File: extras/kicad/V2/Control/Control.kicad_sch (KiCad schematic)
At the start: 41 parts, among them J1 Ultrasonic Ranging, J2 Conn_01x05, J3 Output, J4 Input, J6 left, J7 right, P8 BeagleBone_Black_Header, P9 BeagleBone_Black_Header, U1 SparkFun-micromod, U2 ESP-01-WIFI, U3 LIS3DHTR, U4 BNO085-breackout, U6 PCA9557PW

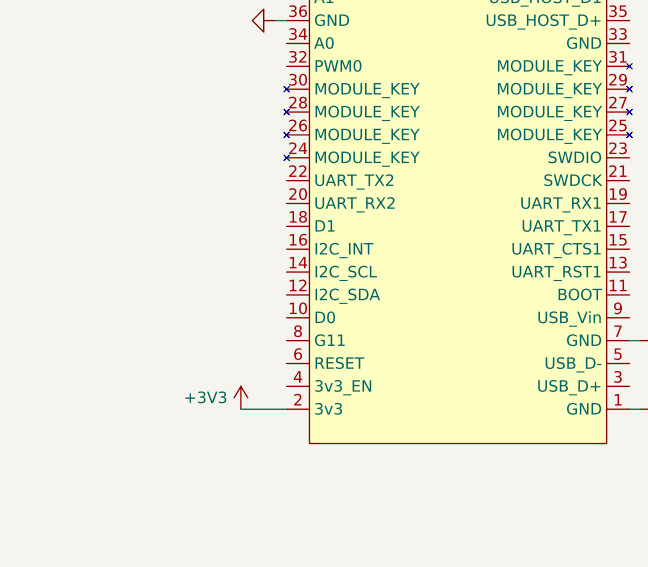
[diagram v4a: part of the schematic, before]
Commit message: f
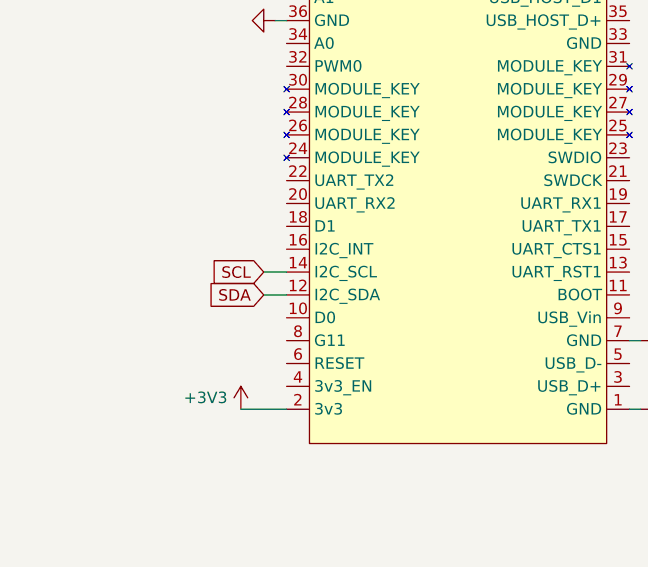
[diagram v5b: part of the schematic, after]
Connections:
- net SCL: now also U1.14 (I2C_SCL)
- net SDA: now also U1.12 (I2C_SDA)
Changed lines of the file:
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@@
+    (stroke (width 0) (type default) (color 0 0 0 0))
+  )
+  (wire (pts (xy 53.34 130.81) (xy 50.8 130.81))
     (stroke (width 0) (type default) (color 0 0 0 0))
   )
@@
   )
   (wire (pts (xy 189.23 102.87) (xy 193.04 102.87))
+    (stroke (width 0) (type default) (color 0 0 0 0))
+  )
+  (wire (pts (xy 53.34 133.35) (xy 50.8 133.35))
     (stroke (width 0) (type default) (color 0 0 0 0))
   )
@@
     )
   )
+  (global_label "SCL" (shape input) (at 50.8 130.81 180) (fields_autoplaced)
+    (effects (font (size 1.27 1.27)) (justify right))
+    (property "Intersheet References" "${INTERSHEET_REFS}" (id 0) (at 44.8793 130.7306 0)
+      (effects (font (size 1.27 1.27)) (justify right) hide)
+    )
+  )
   (global_label "SDA" (shape input) (at 480.06 122.555 180) (fields_autoplaced)
     (effects (font (size 1.27 1.27)) (justify right))
@@
       (effects (font (size 1.27 1.27)) (justify right) hide)
     )
+  )
+  (global_label "SDA" (shape input) (at 50.8 133.35 180) (fields_autoplaced)
+    (effects (font (size 1.27 1.27)) (justify right))
+    (property "Intersheet References" "${INTERSHEET_REFS}" (id 0) (at 44.8188 133.2706 0)
+      (effects (font (size 1.27 1.27)) (justify right) hide)
+    )
